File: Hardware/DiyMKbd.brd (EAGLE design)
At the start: 83 x 98 mm, 68 parts

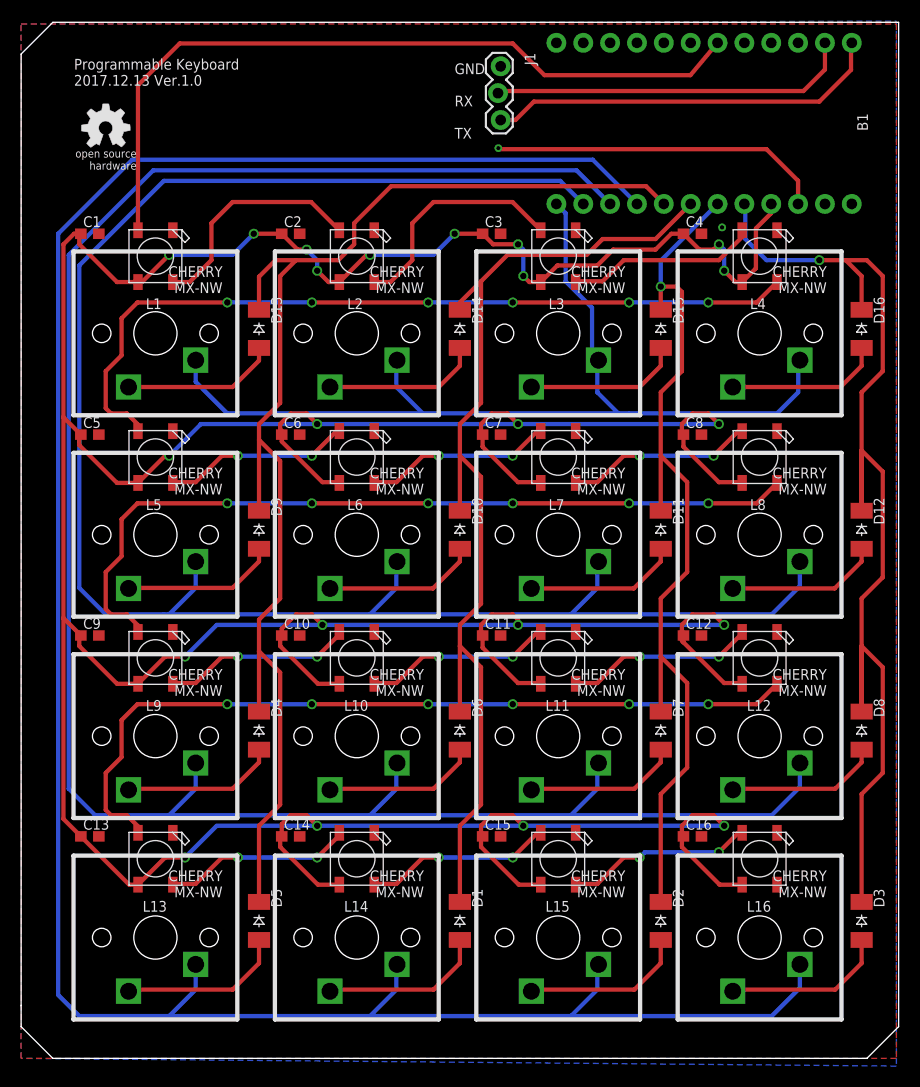
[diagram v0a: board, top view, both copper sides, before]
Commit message: add gerber file
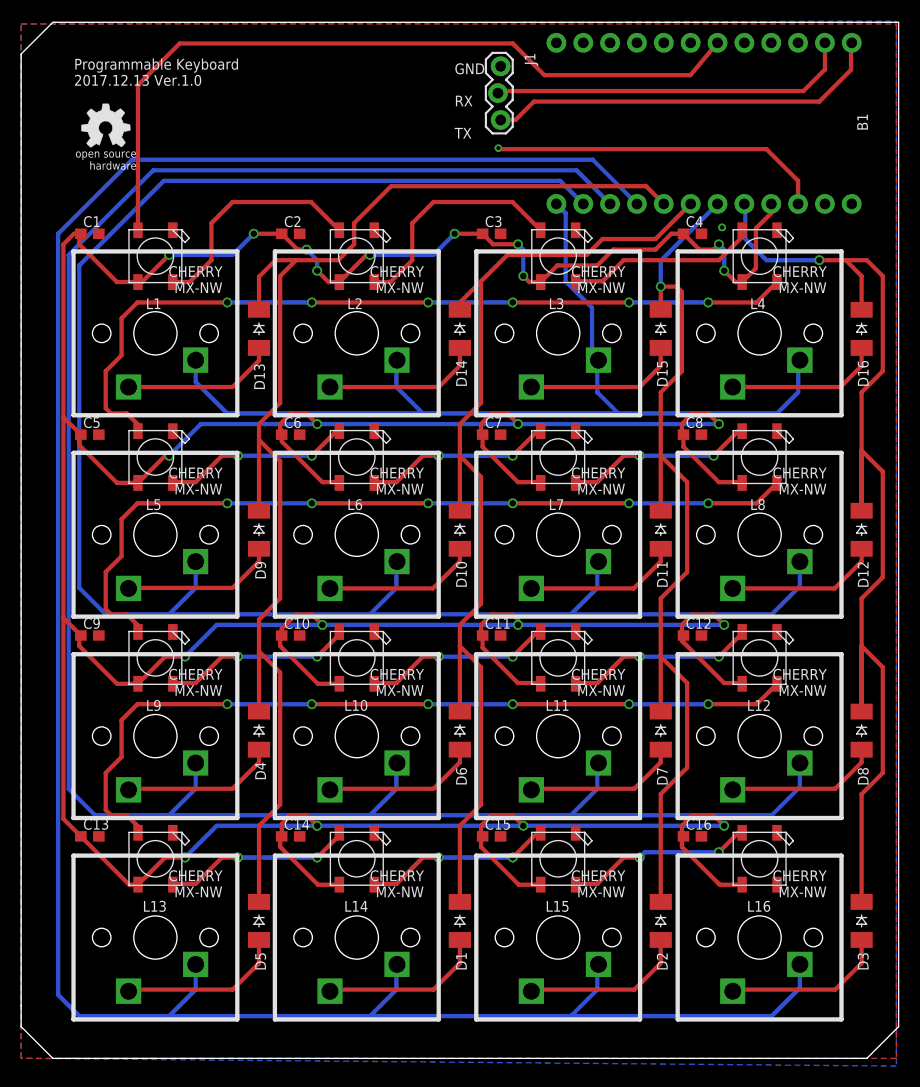
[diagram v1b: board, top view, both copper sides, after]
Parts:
- J1: value (none) -> 2.54 header
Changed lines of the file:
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@@
 <setting verticaltext="up"/>
 </settings>
-<grid distance="1" unitdist="mm" unit="mm" style="lines" multiple="1" display="yes" altdistance="0.025" altunitdist="inch" altunit="mm"/>
+<grid distance="0.5" unitdist="mm" unit="mm" style="lines" multiple="1" display="yes" altdistance="0.025" altunitdist="inch" altunit="mm"/>
 <layers>
 <layer number="1" name="Top" color="4" fill="1" visible="yes" active="yes"/>
@@
 <attribute name="VALUE" x="49.106" y="88.44" size="0.6096" layer="27" font="vector" ratio="20" rot="R270" align="top-center"/>
 </element>
-<element name="J1" library="SparkFun-Connectors" package="1X03_LOCK" value="" x="45.23" y="93.84" smashed="yes" rot="R270">
+<element name="J1" library="SparkFun-Connectors" package="1X03_LOCK" value="2.54 header" x="45.23" y="93.84" smashed="yes" rot="R270">
 <attribute name="NAME" x="47.627" y="95.11" size="1.016" layer="25" font="vector" rot="R270"/>
 <attribute name="VALUE" x="43.198" y="95.11" size="0.6096" layer="27" font="vector" ratio="20" rot="R270"/>
@@
 </element>
 <element name="D5" library="diode" package="SOD-123_MINI-SMA" value="CGRM4001-G" x="22.5" y="13" smashed="yes" rot="R270">
-<attribute name="NAME" x="23.643" y="16.048" size="1.016" layer="25" font="vector" rot="R270"/>
+<attribute name="NAME" x="22.143" y="10.048" size="1.016" layer="25" font="vector" rot="R270"/>
 <attribute name="VALUE" x="20.087" y="16.048" size="1.27" layer="27" rot="R270"/>
 </element>
 <element name="D1" library="diode" package="SOD-123_MINI-SMA" value="CGRM4001-G" x="41.5" y="13" smashed="yes" rot="R270">
-<attribute name="NAME" x="42.643" y="16.048" size="1.016" layer="25" font="vector" rot="R270"/>
+<attribute name="NAME" x="41.143" y="10.048" size="1.016" layer="25" font="vector" rot="R270"/>
 <attribute name="VALUE" x="39.087" y="16.048" size="1.27" layer="27" rot="R270"/>
 </element>
 <element name="D2" library="diode" package="SOD-123_MINI-SMA" value="CGRM4001-G" x="60.5" y="13" smashed="yes" rot="R270">
-<attribute name="NAME" x="61.643" y="16.048" size="1.016" layer="25" font="vector" rot="R270"/>
+<attribute name="NAME" x="60.143" y="10.048" size="1.016" layer="25" font="vector" rot="R270"/>
 <attribute name="VALUE" x="58.087" y="16.048" size="1.27" layer="27" rot="R270"/>
 </element>
 <element name="D3" library="diode" package="SOD-123_MINI-SMA" value="CGRM4001-G" x="79.5" y="13" smashed="yes" rot="R270">
-<attribute name="NAME" x="80.643" y="16.048" size="1.016" layer="25" font="vector" rot="R270"/>
+<attribute name="NAME" x="79.143" y="10.048" size="1.016" layer="25" font="vector" rot="R270"/>
 <attribute name="VALUE" x="77.087" y="16.048" size="1.27" layer="27" rot="R270"/>
 </element>
 <element name="D4" library="diode" package="SOD-123_MINI-SMA" value="CGRM4001-G" x="22.5" y="31" smashed="yes" rot="R270">
-<attribute name="NAME" x="23.643" y="34.048" size="1.016" layer="25" font="vector" rot="R270"/>
+<attribute name="NAME" x="22.143" y="28.048" size="1.016" layer="25" font="vector" rot="R270"/>
 <attribute name="VALUE" x="20.087" y="34.048" size="1.27" layer="27" rot="R270"/>
 </element>
 <element name="D6" library="diode" package="SOD-123_MINI-SMA" value="CGRM4001-G" x="41.5" y="31" smashed="yes" rot="R270">
-<attribute name="NAME" x="42.643" y="34.048" size="1.016" layer="25" font="vector" rot="R270"/>
+<attribute name="NAME" x="41.143" y="27.548" size="1.016" layer="25" font="vector" rot="R270"/>
 <attribute name="VALUE" x="39.087" y="34.048" size="1.27" layer="27" rot="R270"/>
 </element>
 <element name="D7" library="diode" package="SOD-123_MINI-SMA" value="CGRM4001-G" x="60.5" y="31" smashed="yes" rot="R270">
-<attribute name="NAME" x="61.643" y="34.048" size="1.016" layer="25" font="vector" rot="R270"/>
+<attribute name="NAME" x="60.143" y="27.548" size="1.016" layer="25" font="vector" rot="R270"/>
 <attribute name="VALUE" x="58.087" y="34.048" size="1.27" layer="27" rot="R270"/>
 </element>
 <element name="D8" library="diode" package="SOD-123_MINI-SMA" value="CGRM4001-G" x="79.5" y="31" smashed="yes" rot="R270">
-<attribute name="NAME" x="80.643" y="34.048" size="1.016" layer="25" font="vector" rot="R270"/>
+<attribute name="NAME" x="79.143" y="27.548" size="1.016" layer="25" font="vector" rot="R270"/>
 <attribute name="VALUE" x="77.087" y="34.048" size="1.27" layer="27" rot="R270"/>
 </element>
 <element name="D9" library="diode" package="SOD-123_MINI-SMA" value="CGRM4001-G" x="22.5" y="50" smashed="yes" rot="R270">
-<attribute name="NAME" x="23.643" y="53.048" size="1.016" layer="25" font="vector" rot="R270"/>
+<attribute name="NAME" x="22.143" y="47.048" size="1.016" layer="25" font="vector" rot="R270"/>
 <attribute name="VALUE" x="20.087" y="53.048" size="1.27" layer="27" rot="R270"/>
 </element>
 <element name="D10" library="diode" package="SOD-123_MINI-SMA" value="CGRM4001-G" x="41.5" y="50" smashed="yes" rot="R270">
-<attribute name="NAME" x="42.643" y="53.048" size="1.016" layer="25" font="vector" rot="R270"/>
+<attribute name="NAME" x="41.143" y="47.048" size="1.016" layer="25" font="vector" rot="R270"/>
 <attribute name="VALUE" x="39.087" y="53.048" size="1.27" layer="27" rot="R270"/>
 </element>
 <element name="D11" library="diode" package="SOD-123_MINI-SMA" value="CGRM4001-G" x="60.5" y="50" smashed="yes" rot="R270">
-<attribute name="NAME" x="61.643" y="53.048" size="1.016" layer="25" font="vector" rot="R270"/>
+<attribute name="NAME" x="60.143" y="47.048" size="1.016" layer="25" font="vector" rot="R270"/>
 <attribute name="VALUE" x="58.087" y="53.048" size="1.27" layer="27" rot="R270"/>
 </element>
 <element name="D12" library="diode" package="SOD-123_MINI-SMA" value="CGRM4001-G" x="79.5" y="50" smashed="yes" rot="R270">
-<attribute name="NAME" x="80.643" y="53.048" size="1.016" layer="25" font="vector" rot="R270"/>
+<attribute name="NAME" x="79.143" y="47.048" size="1.016" layer="25" font="vector" rot="R270"/>
 <attribute name="VALUE" x="77.087" y="53.048" size="1.27" layer="27" rot="R270"/>
 </element>
 <element name="D13" library="diode" package="SOD-123_MINI-SMA" value="CGRM4001-G" x="22.5" y="69" smashed="yes" rot="R270">
-<attribute name="NAME" x="23.643" y="72.048" size="1.016" layer="25" font="vector" rot="R270"/>
+<attribute name="NAME" x="22.043" y="65.748" size="1.016" layer="25" font="vector" rot="R270"/>
 <attribute name="VALUE" x="20.087" y="72.048" size="1.27" layer="27" rot="R270"/>
 </element>
 <element name="D14" library="diode" package="SOD-123_MINI-SMA" value="CGRM4001-G" x="41.5" y="69" smashed="yes" rot="R270">
-<attribute name="NAME" x="42.643" y="72.048" size="1.016" layer="25" font="vector" rot="R270"/>
+<attribute name="NAME" x="41.143" y="66.048" size="1.016" layer="25" font="vector" rot="R270"/>
 <attribute name="VALUE" x="39.087" y="72.048" size="1.27" layer="27" rot="R270"/>
 </element>
 <element name="D15" library="diode" package="SOD-123_MINI-SMA" value="CGRM4001-G" x="60.5" y="69" smashed="yes" rot="R270">
-<attribute name="NAME" x="61.643" y="72.048" size="1.016" layer="25" font="vector" rot="R270"/>
+<attribute name="NAME" x="60.143" y="66.048" size="1.016" layer="25" font="vector" rot="R270"/>
 <attribute name="VALUE" x="58.087" y="72.048" size="1.27" layer="27" rot="R270"/>
 </element>
 <element name="D16" library="diode" package="SOD-123_MINI-SMA" value="CGRM4001-G" x="79.5" y="69" smashed="yes" rot="R270">
-<attribute name="NAME" x="80.643" y="72.048" size="1.016" layer="25" font="vector" rot="R270"/>
+<attribute name="NAME" x="79.143" y="66.048" size="1.016" layer="25" font="vector" rot="R270"/>
 <attribute name="VALUE" x="77.087" y="72.048" size="1.27" layer="27" rot="R270"/>
 </element>
